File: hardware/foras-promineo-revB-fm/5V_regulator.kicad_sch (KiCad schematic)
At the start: 15 parts, among them Q222 MMBT3906-7-F, U210 TPS63070

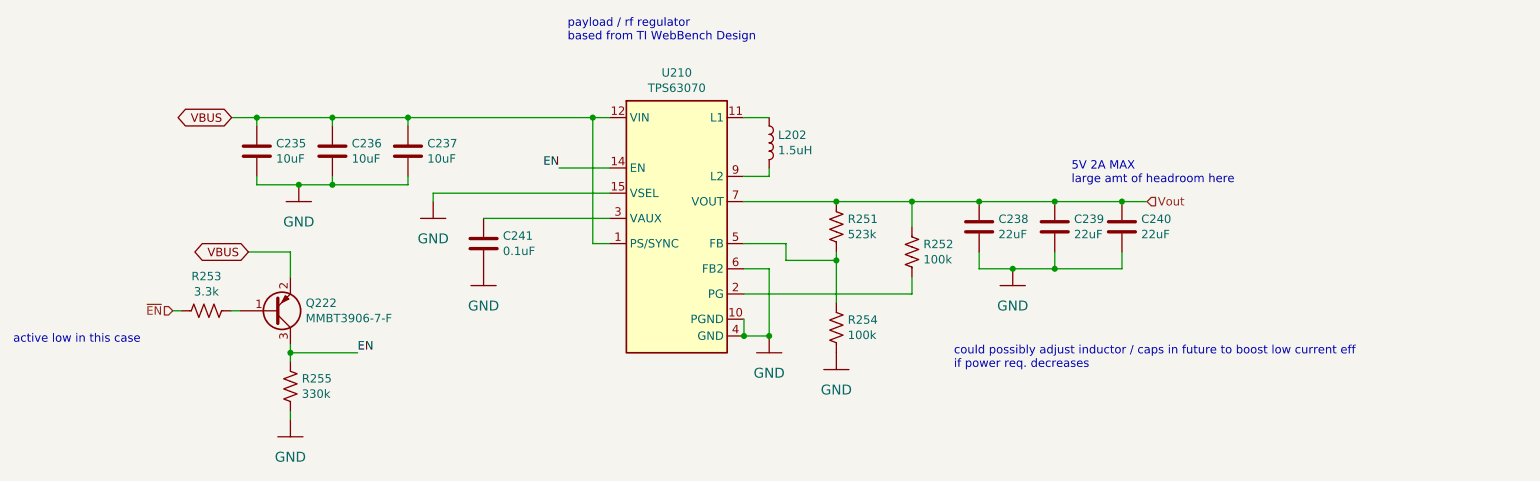
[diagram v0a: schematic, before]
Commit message: added charge current monitor
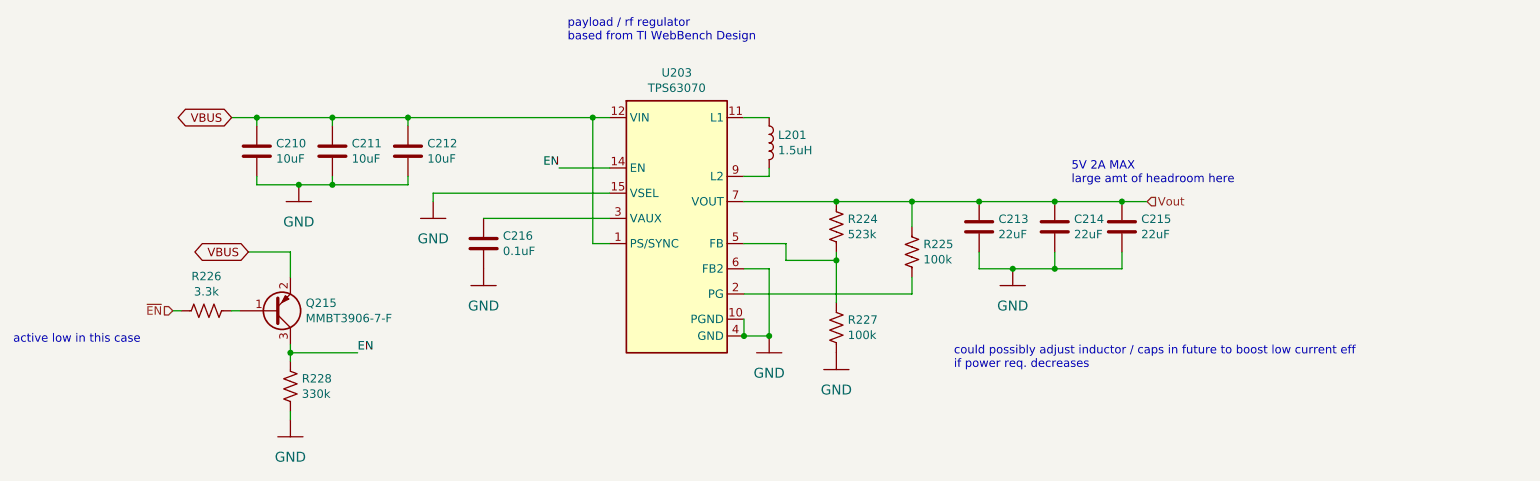
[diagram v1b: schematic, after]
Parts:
- renumbered C235 to C210, C236 to C211, C237 to C212, C238 to C213, C239 to C214, C240 to C215, C241 to C216, L202 to L201, Q222 to Q215, R251 to R224, R252 to R225, R253 to R226, R254 to R227, R255 to R228, U210 to U203
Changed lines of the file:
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@@
     (effects (font (size 1.27 1.27)) (justify right))
   )
-  (symbol (lib_id "mainboard_SLI:TPS63070") (at 156.21 58.42 0) (unit 1)
-    (in_bom yes) (on_board yes)
-    (property "Reference" "U210" (id 0) (at 156.21 41.4782 0))
+  (symbol (lib_id "mainboard_SLI:TPS63070") (at 156.21 58.42 0)
+    (in_bom yes) (on_board yes)
+    (property "Reference" "U203" (id 0) (at 156.21 41.4782 0))
     (property "Value" "TPS63070" (id 1) (at 156.21 43.7896 0))
     (property "Footprint" "mainboard-SLI:TPS63070RNMR" (id 2) (at 157.48 85.09 0)
@@
     (pin "9")
   )
-  (symbol (lib_id "mainboard-rescue:R_US-Device-mainboard-rescue") (at 97.79 88.9 0) (unit 1)
-    (in_bom yes) (on_board yes)
-    (property "Reference" "R255" (id 0) (at 99.5172 87.7316 0)
+  (symbol (lib_id "mainboard-rescue:R_US-Device-mainboard-rescue") (at 97.79 88.9 0)
+    (in_bom yes) (on_board yes)
+    (property "Reference" "R228" (id 0) (at 99.5172 87.7316 0)
       (effects (font (size 1.27 1.27)) (justify left))
     )
@@
     (pin "2")
   )
-  (symbol (lib_id "mainboard:GND") (at 127 73.66 0) (unit 1)
-    (in_bom yes) (on_board yes)
-    (property "Reference" "#GND0159" (id 0) (at 127 73.66 0)
+  (symbol (lib_id "mainboard:GND") (at 127 73.66 0)
+    (in_bom yes) (on_board yes)
+    (property "Reference" "#GND0118" (id 0) (at 127 73.66 0)
       (effects (font (size 1.27 1.27)) hide)
     )
@@
     (pin "1")
   )
-  (symbol (lib_id "mainboard-rescue:C-Device-mainboard-rescue") (at 127 67.31 180) (unit 1)
-    (in_bom yes) (on_board yes)
-    (property "Reference" "C241" (id 0) (at 129.921 66.1416 0)
+  (symbol (lib_id "mainboard-rescue:C-Device-mainboard-rescue") (at 127 67.31 180)
+    (in_bom yes) (on_board yes)
+    (property "Reference" "C216" (id 0) (at 129.921 66.1416 0)
       (effects (font (size 1.27 1.27)) (justify right))
     )
@@
     (pin "2")
   )
-  (symbol (lib_id "mainboard-rescue:C-Device-mainboard-rescue") (at 115.57 53.34 0) (unit 1)
-    (in_bom yes) (on_board yes)
-    (property "Reference" "C237" (id 0) (at 118.491 52.1716 0)
+  (symbol (lib_id "mainboard-rescue:C-Device-mainboard-rescue") (at 115.57 53.34 0)
+    (in_bom yes) (on_board yes)
+    (property "Reference" "C212" (id 0) (at 118.491 52.1716 0)
       (effects (font (size 1.27 1.27)) (justify left))
     )
@@
     (pin "2")
   )
-  (symbol (lib_id "mainboard-rescue:C-Device-mainboard-rescue") (at 104.14 53.34 0) (unit 1)
-    (in_bom yes) (on_board yes)
-    (property "Reference" "C236" (id 0) (at 107.061 52.1716 0)
+  (symbol (lib_id "mainboard-rescue:C-Device-mainboard-rescue") (at 104.14 53.34 0)
+    (in_bom yes) (on_board yes)
+    (property "Reference" "C211" (id 0) (at 107.061 52.1716 0)
       (effects (font (size 1.27 1.27)) (justify left))
     )
@@
     (pin "2")
   )
-  (symbol (lib_id "mainboard-rescue:C-Device-mainboard-rescue") (at 92.71 53.34 0) (unit 1)
-    (in_bom yes) (on_board yes)
-    (property "Reference" "C235" (id 0) (at 95.631 52.1716 0)
+  (symbol (lib_id "mainboard-rescue:C-Device-mainboard-rescue") (at 92.71 53.34 0)
+    (in_bom yes) (on_board yes)
+    (property "Reference" "C210" (id 0) (at 95.631 52.1716 0)
       (effects (font (size 1.27 1.27)) (justify left))
     )
@@
     (pin "2")
   )
-  (symbol (lib_id "mainboard:GND") (at 99.06 60.96 0) (unit 1)
-    (in_bom yes) (on_board yes)
-    (property "Reference" "#GND0160" (id 0) (at 99.06 60.96 0)
+  (symbol (lib_id "mainboard:GND") (at 99.06 60.96 0)
+    (in_bom yes) (on_board yes)
+    (property "Reference" "#GND0119" (id 0) (at 99.06 60.96 0)
       (effects (font (size 1.27 1.27)) hide)
     )
@@
     (pin "1")
   )
-  (symbol (lib_id "mainboard:GND") (at 119.38 63.5 0) (unit 1)
-    (in_bom yes) (on_board yes)
-    (property "Reference" "#GND0161" (id 0) (at 119.38 63.5 0)
+  (symbol (lib_id "mainboard:GND") (at 119.38 63.5 0)
+    (in_bom yes) (on_board yes)
+    (property "Reference" "#GND0125" (id 0) (at 119.38 63.5 0)
       (effects (font (size 1.27 1.27)) hide)
     )
@@
     (pin "1")
   )
-  (symbol (lib_id "mainboard-rescue:L-Device-mainboard-rescue") (at 170.18 52.07 0) (unit 1)
-    (in_bom yes) (on_board yes)
-    (property "Reference" "L202" (id 0) (at 171.5262 50.9016 0)
+  (symbol (lib_id "mainboard-rescue:L-Device-mainboard-rescue") (at 170.18 52.07 0)
+    (in_bom yes) (on_board yes)
+    (property "Reference" "L201" (id 0) (at 171.5262 50.9016 0)
       (effects (font (size 1.27 1.27)) (justify left))
     )
@@
     (pin "2")
   )
-  (symbol (lib_id "mainboard-rescue:R_US-Device-mainboard-rescue") (at 180.34 64.77 0) (unit 1)
-    (in_bom yes) (on_board yes)
-    (property "Reference" "R251" (id 0) (at 182.0672 63.6016 0)
+  (symbol (lib_id "mainboard-rescue:R_US-Device-mainboard-rescue") (at 180.34 64.77 0)
+    (in_bom yes) (on_board yes)
+    (property "Reference" "R224" (id 0) (at 182.0672 63.6016 0)
       (effects (font (size 1.27 1.27)) (justify left))
     )
@@
     (pin "2")
   )
-  (symbol (lib_id "mainboard-rescue:R_US-Device-mainboard-rescue") (at 180.34 80.01 0) (unit 1)
-    (in_bom yes) (on_board yes)
-    (property "Reference" "R254" (id 0) (at 182.0672 78.8416 0)
+  (symbol (lib_id "mainboard-rescue:R_US-Device-mainboard-rescue") (at 180.34 80.01 0)
+    (in_bom yes) (on_board yes)
+    (property "Reference" "R227" (id 0) (at 182.0672 78.8416 0)
       (effects (font (size 1.27 1.27)) (justify left))
     )
@@
     (pin "2")
   )
-  (symbol (lib_id "mainboard:GND") (at 180.34 86.36 0) (unit 1)
-    (in_bom yes) (on_board yes)
-    (property "Reference" "#GND0162" (id 0) (at 180.34 86.36 0)
+  (symbol (lib_id "mainboard:GND") (at 180.34 86.36 0)
+    (in_bom yes) (on_board yes)
+    (property "Reference" "#GND0128" (id 0) (at 180.34 86.36 0)
       (effects (font (size 1.27 1.27)) hide)
     )
@@
     (pin "1")
   )
-  (symbol (lib_id "mainboard:GND") (at 170.18 83.82 0) (unit 1)
-    (in_bom yes) (on_board yes)
-    (property "Reference" "#GND0163" (id 0) (at 170.18 83.82 0)
+  (symbol (lib_id "mainboard:GND") (at 170.18 83.82 0)
+    (in_bom yes) (on_board yes)
+    (property "Reference" "#GND0129" (id 0) (at 170.18 83.82 0)
       (effects (font (size 1.27 1.27)) hide)
     )
@@
     (pin "1")
   )
-  (symbol (lib_id "mainboard-rescue:R_US-Device-mainboard-rescue") (at 191.77 68.58 0) (unit 1)
-    (in_bom yes) (on_board yes)
-    (property "Reference" "R252" (id 0) (at 193.4972 67.4116 0)
+  (symbol (lib_id "mainboard-rescue:R_US-Device-mainboard-rescue") (at 191.77 68.58 0)
+    (in_bom yes) (on_board yes)
+    (property "Reference" "R225" (id 0) (at 193.4972 67.4116 0)
       (effects (font (size 1.27 1.27)) (justify left))
     )
@@
     (pin "2")
   )
-  (symbol (lib_id "mainboard-rescue:C-Device-mainboard-rescue") (at 201.93 64.77 0) (unit 1)
-    (in_bom yes) (on_board yes)
-    (property "Reference" "C238" (id 0) (at 204.851 63.6016 0)
+  (symbol (lib_id "mainboard-rescue:C-Device-mainboard-rescue") (at 201.93 64.77 0)
+    (in_bom yes) (on_board yes)
+    (property "Reference" "C213" (id 0) (at 204.851 63.6016 0)
       (effects (font (size 1.27 1.27)) (justify left))
     )
@@
     (pin "2")
   )
-  (symbol (lib_id "mainboard-rescue:C-Device-mainboard-rescue") (at 213.36 64.77 0) (unit 1)
-    (in_bom yes) (on_board yes)
-    (property "Reference" "C239" (id 0) (at 216.281 63.6016 0)
+  (symbol (lib_id "mainboard-rescue:C-Device-mainboard-rescue") (at 213.36 64.77 0)
+    (in_bom yes) (on_board yes)
+    (property "Reference" "C214" (id 0) (at 216.281 63.6016 0)
       (effects (font (size 1.27 1.27)) (justify left))
     )
@@
     (pin "2")
   )
-  (symbol (lib_id "mainboard:GND") (at 207.01 73.66 0) (unit 1)
-    (in_bom yes) (on_board yes)
-    (property "Reference" "#GND0164" (id 0) (at 207.01 73.66 0)
+  (symbol (lib_id "mainboard:GND") (at 207.01 73.66 0)
+    (in_bom yes) (on_board yes)
+    (property "Reference" "#GND0130" (id 0) (at 207.01 73.66 0)
       (effects (font (size 1.27 1.27)) hide)
     )
@@
     (pin "1")
   )
-  (symbol (lib_id "mainboard-rescue:C-Device-mainboard-rescue") (at 223.52 64.77 0) (unit 1)
-    (in_bom yes) (on_board yes)
-    (property "Reference" "C240" (id 0) (at 226.441 63.6016 0)
+  (symbol (lib_id "mainboard-rescue:C-Device-mainboard-rescue") (at 223.52 64.77 0)
+    (in_bom yes) (on_board yes)
+    (property "Reference" "C215" (id 0) (at 226.441 63.6016 0)
       (effects (font (size 1.27 1.27)) (justify left))
     )
@@
     (pin "2")
   )
-  (symbol (lib_id "mainboard-rescue:Q_PNP_BEC-Device-mainboard-rescue") (at 95.25 77.47 0) (mirror x) (unit 1)
-    (in_bom yes) (on_board yes)
-    (property "Reference" "Q222" (id 0) (at 100.1014 76.3016 0)
+  (symbol (lib_id "mainboard-rescue:Q_PNP_BEC-Device-mainboard-rescue") (at 95.25 77.47 0) (mirror x)
+    (in_bom yes) (on_board yes)
+    (property "Reference" "Q215" (id 0) (at 100.1014 76.3016 0)
       (effects (font (size 1.27 1.27)) (justify left))
     )
@@
     (pin "3")
   )
-  (symbol (lib_id "mainboard:GND") (at 97.79 96.52 0) (unit 1)
-    (in_bom yes) (on_board yes)
-    (property "Reference" "#GND0165" (id 0) (at 97.79 96.52 0)
+  (symbol (lib_id "mainboard:GND") (at 97.79 96.52 0)
+    (in_bom yes) (on_board yes)
+    (property "Reference" "#GND0131" (id 0) (at 97.79 96.52 0)
       (effects (font (size 1.27 1.27)) hide)
     )
@@
     (pin "1")
   )
-  (symbol (lib_id "mainboard-rescue:R_US-Device-mainboard-rescue") (at 85.09 77.47 270) (unit 1)
-    (in_bom yes) (on_board yes)
-    (property "Reference" "R253" (id 0) (at 85.09 72.263 90))
+  (symbol (lib_id "mainboard-rescue:R_US-Device-mainboard-rescue") (at 85.09 77.47 270)
+    (in_bom yes) (on_board yes)
+    (property "Reference" "R226" (id 0) (at 85.09 72.263 90))
     (property "Value" "3.3k" (id 1) (at 85.09 74.5744 90))
     (property "Footprint" "Resistor_SMD:R_0603_1608Metric" (id 2) (at 84.836 78.486 90)
